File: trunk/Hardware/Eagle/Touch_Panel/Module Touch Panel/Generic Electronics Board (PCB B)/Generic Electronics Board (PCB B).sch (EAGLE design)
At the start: 54 parts, among them IC1 ST3485, IC3 DS18B20, U1 XMEGA-A4TQFP, U2 SPX1117M3-L-3-3, X1 RJ45-8L-B, X6 RJ45-8L-B

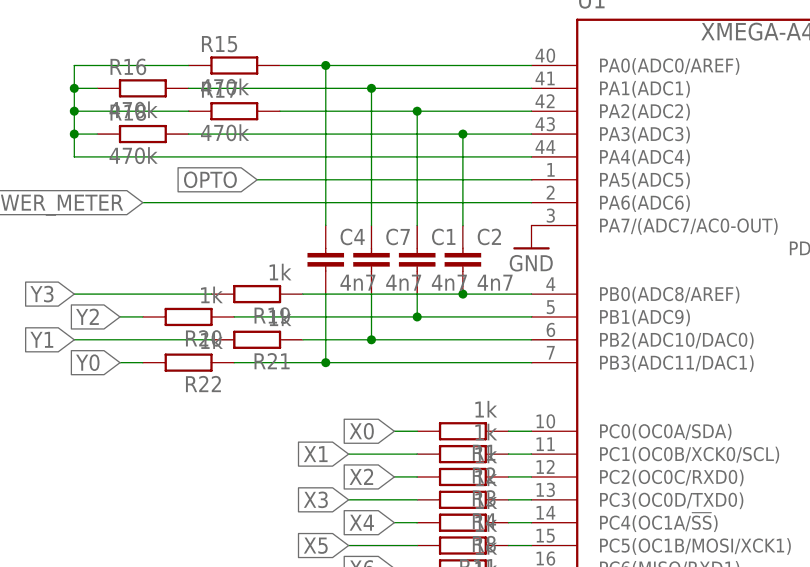
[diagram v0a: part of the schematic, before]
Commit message: Minor changes
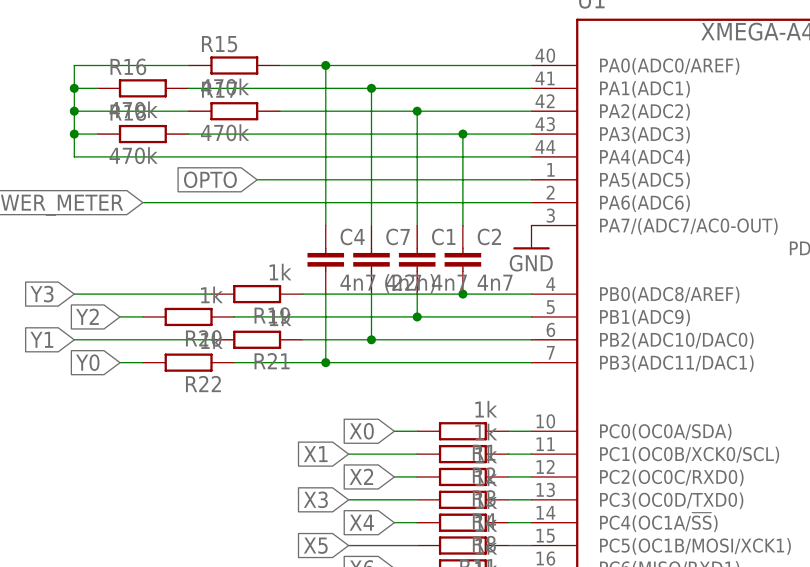
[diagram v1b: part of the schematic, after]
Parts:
- C4: value 4n7 -> 4n7 (22n)
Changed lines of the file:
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@@
 <part name="R14" library="rcl" deviceset="R-EU_" device="R0603" value="1k"/>
 <part name="C1" library="rcl" deviceset="C-EU" device="C0603" value="4n7"/>
-<part name="C4" library="rcl" deviceset="C-EU" device="C0603" value="4n7"/>
+<part name="C4" library="rcl" deviceset="C-EU" device="C0603" value="4n7 (22n)"/>
 <part name="C7" library="rcl" deviceset="C-EU" device="C0603" value="4n7"/>
 <part name="GND1" library="supply1" deviceset="GND" device=""/>
